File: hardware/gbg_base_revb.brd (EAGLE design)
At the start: 50 x 34.5 mm, 15 parts, among them Q3 NTS4173, U1 AB0805, U2 USD-SOCKET, U3 LP2985AIM5-3.3

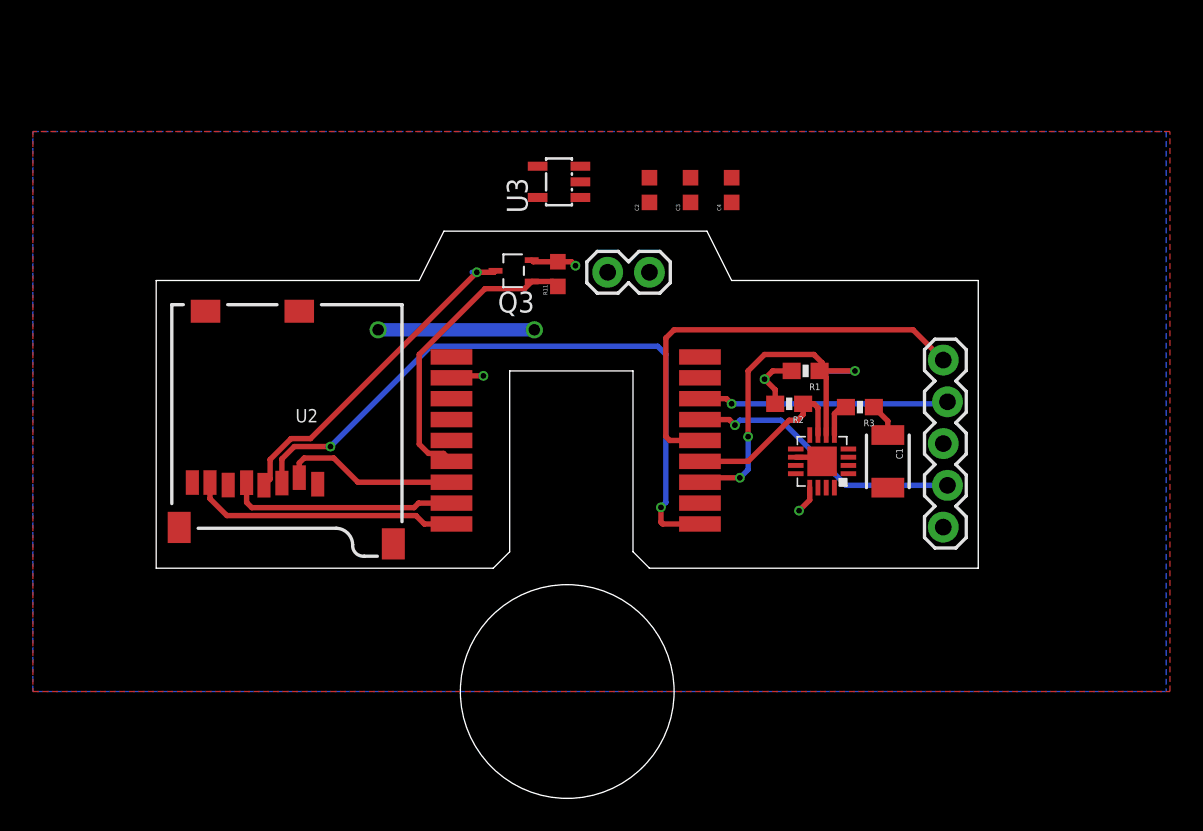
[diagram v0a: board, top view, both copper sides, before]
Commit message: new hardware, simple
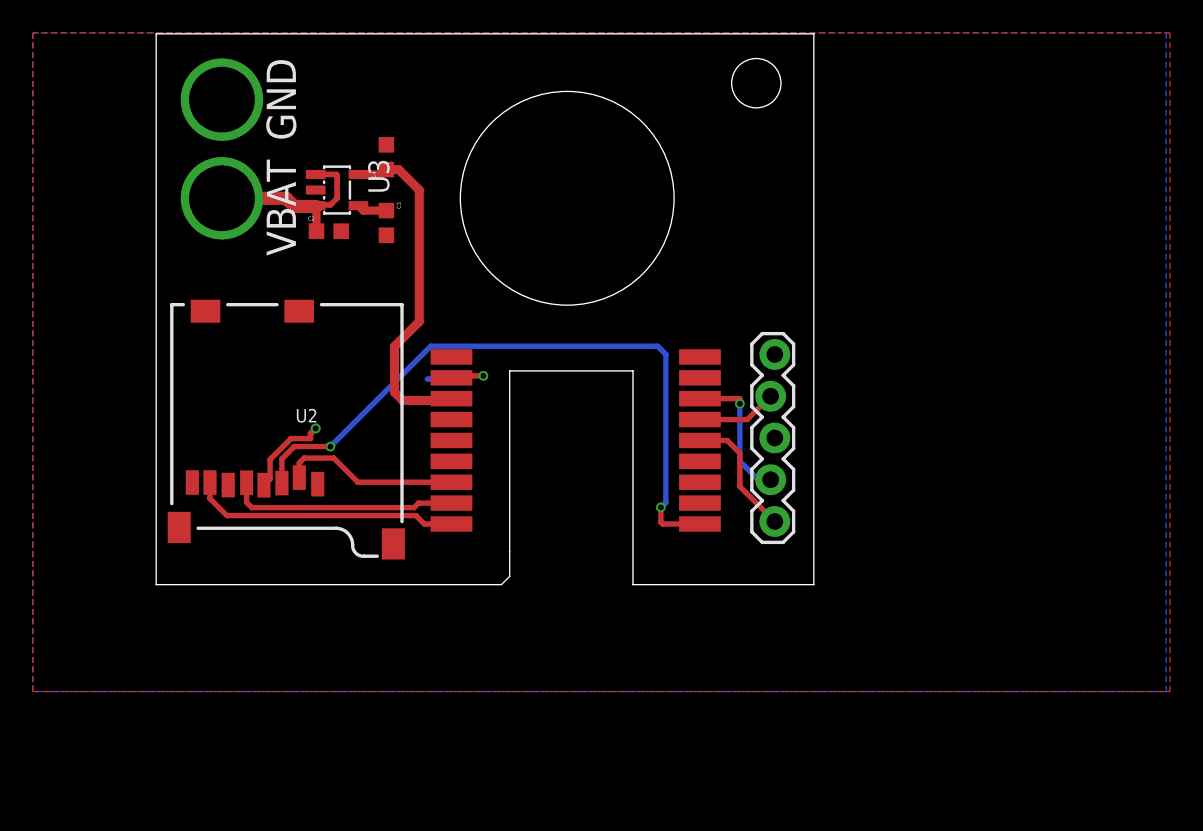
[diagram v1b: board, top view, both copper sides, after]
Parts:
- removed C1: (no value), SparkFun-Passives:1210
- removed JP1: (no value), SparkFun-Connectors:1X02
- removed Q3: NTS4173, nts4173p:SC-70-3
- removed R1, R2: 4.7k, SparkFun-Resistors:0603-RES
- removed R11: 220k, tiny_passives:0603
- removed R3: 1.5k, SparkFun-Resistors:0603-RES
- removed U1: AB0805, AB08XX:QFN16
- moved C4 21.1 mm to (21.0, 32.5)
- moved C2 19.7 mm to (17.5, 28.0), turned to 0 degrees
- moved C3 18.6 mm to (21.0, 28.5), turned to 270 degrees
- moved JP2 14.8 mm to (44.5, 20.5), turned to 270 degrees
- moved U3 13.5 mm to (18.0, 30.5), turned to 270 degrees
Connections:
- removed net N$1: C1.1, R3.1
- removed net N$5: R3.2, U1.5
- removed net SD_VCC: Q3.P3, U2.4
- net !SD_ENABLE: no longer Q3.P1, R11.1
- net GND: no longer C1.2, JP1.1, U1.10, U1.2, U1.9, U1.TH
- net I2C_SCL: no longer R2.1, U1.7
- net I2C_SDA: no longer R1.1, U1.6
- net VBAT: no longer JP1.2
- net VCC: now also U2.4; no longer Q3.P2, R1.2, R11.2, R2.2, U1.13
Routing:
- net I2C_SDA: track 23.1 -> 0.70 mm, vias 3 -> 0
- net VOUT: track 0.00 -> 21.0 mm
- net SD_VCC: track 20.5 -> 0.00 mm, vias 1 -> 0
- net !SD_ENABLE: track 18.2 -> 0.00 mm
- net RESET: track 26.0 -> 7.79 mm
- net SWDCLK: track 17.0 -> 4.89 mm, vias 1 -> 0
- net VBAT: track 0.00 -> 11.7 mm, vias 0 -> 1
- net GND: track 11.2 -> 0.00 mm, vias 2 -> 1
- net I2C_SCL: track 10.8 -> 0.00 mm
- net SWDIO: track 15.2 -> 8.57 mm
- net N$1: track 2.47 -> 0.00 mm
- net N$5: track 2.15 -> 0.00 mm
- net BYPASS: track 0.00 -> 1.82 mm
- net VCC: track 10.1 -> 8.94 mm, vias 4 -> 2
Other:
- board size 50 x 34.5 mm -> 40 x 33.5 mm
- board text added: ""GBG Based" Rev B. Designed by Josiah Hester Northwestern University"
- board text added: "GND"
- board text added: "VBAT"
- board text removed: ""GBG Based" Rev A. Designed by Josiah Hester Northwestern University"
